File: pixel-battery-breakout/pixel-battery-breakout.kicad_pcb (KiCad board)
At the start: 2 copper layers, 68.8 x 51 mm, 7 parts, among them J1 BATT+, J2 BATT-, J3 GND_SHIELD, J4 Conn_01x02_Female, J5 Conn_01x04_Female

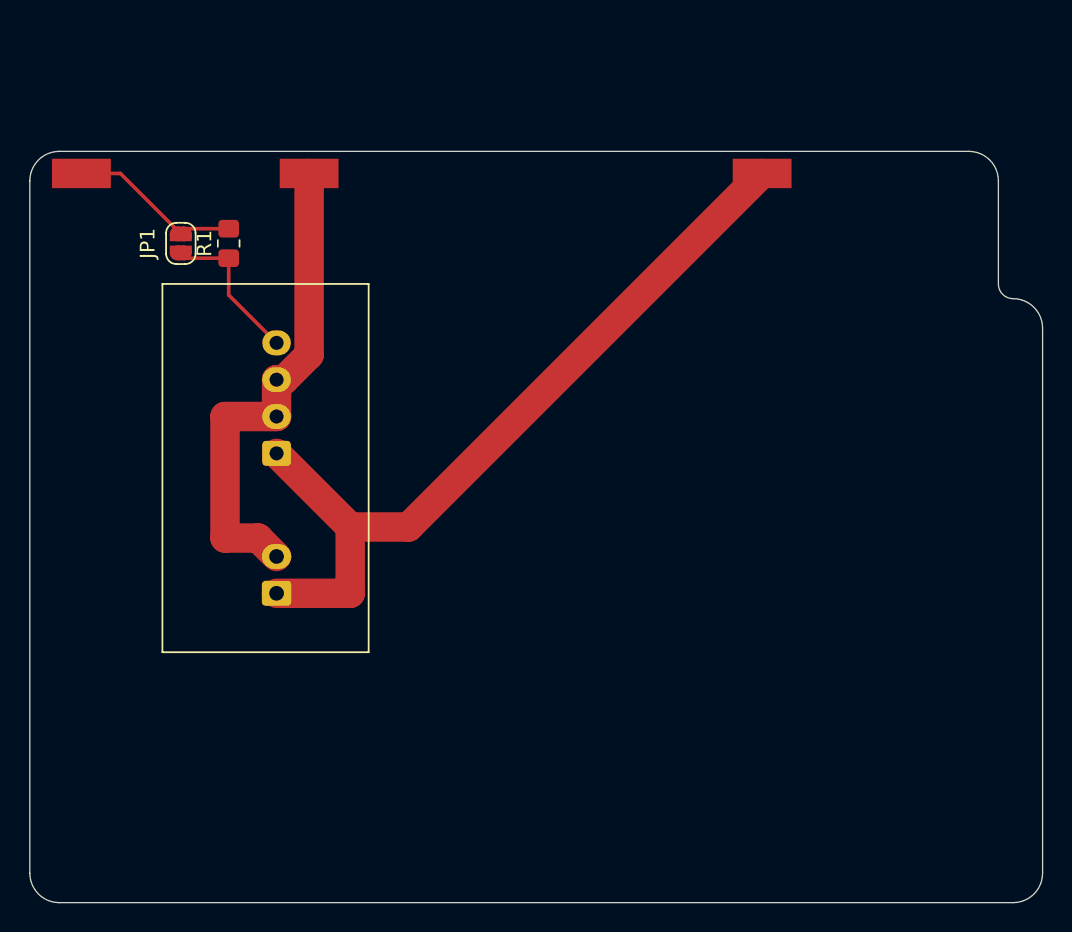
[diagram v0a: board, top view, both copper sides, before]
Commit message: sync
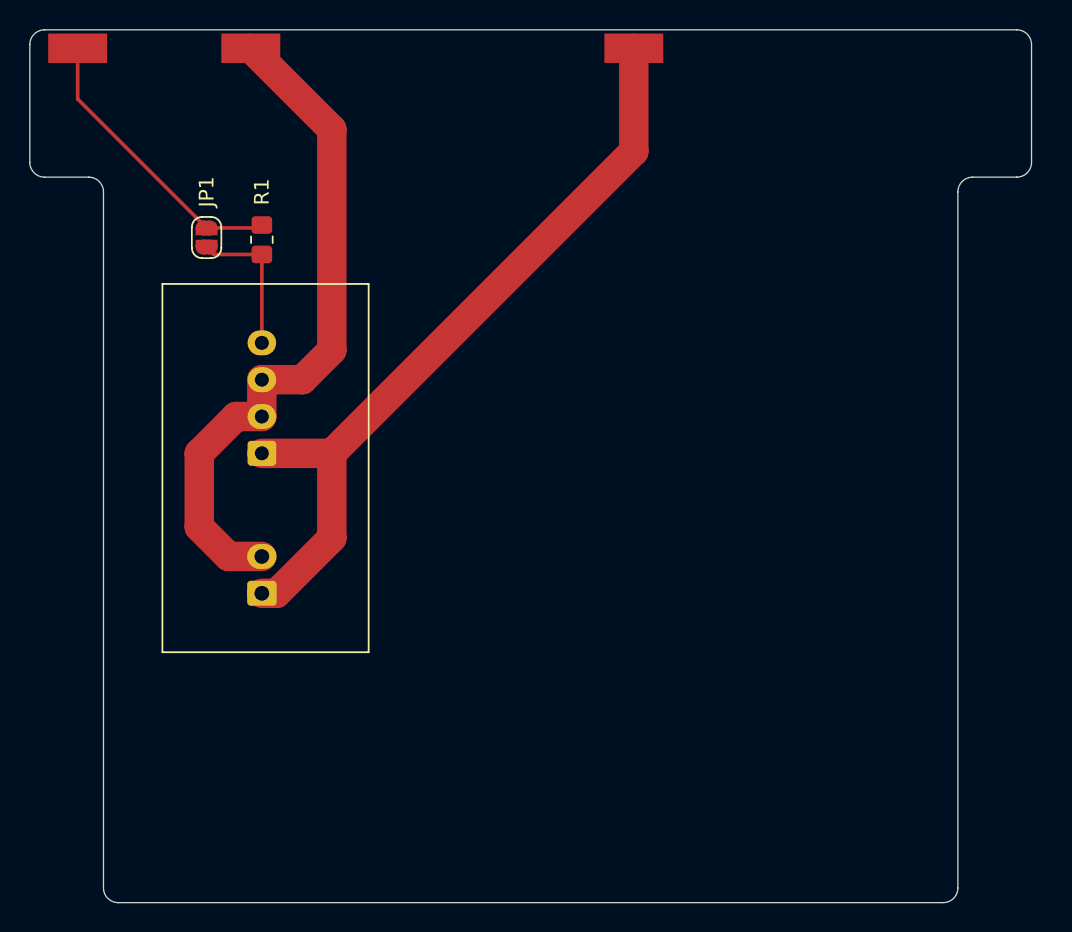
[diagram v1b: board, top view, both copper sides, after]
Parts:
- moved J1 12.2 mm to (176.0, 20.5)
- moved J2 9.38 mm to (150.0, 20.5)
- moved J3 8.50 mm to (138.3, 20.5)
- moved R1 2.26 mm to (148.2, 33.5)
- moved JP1 1.80 mm to (144.5, 33.4)
- moved J4 1.00 mm to (148.2, 57.5)
- moved J5 1.00 mm to (148.2, 48.0)
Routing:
- net Net-(J2-Pad1): track 33.5 -> 46.2 mm
- net Net-(J3-Pad1): track 11.8 -> 19.7 mm
- net Net-(J1-Pad1): track 54.5 -> 52.8 mm
- net Net-(J5-Pad4): track 10.5 -> 9.96 mm
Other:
- board size 68.8 x 51 mm -> 68 x 59.2 mm
- board text added: "SHD"
- board text removed: "SLD"
